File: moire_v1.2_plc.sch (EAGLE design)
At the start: 137 parts, among them IC1 TLC59281DBQ, IC11 LM4040B25, IC2 ROF-78E3.3-0.5SMD, IC3 4051PW, IC4 LM324PW, IC7 LD2981ABU33, IC9 LM324PW, J1 PJ301_THONKICONN6, J10 PJ301_THONKICONN6, J11 PJ301_THONKICONN6, J12 PJ301_THONKICONN6, J2 PJ301_THONKICONN6, J3 PJ301_THONKICONN6, J4 PJ301_THONKICONN6, J5 PJ301_THONKICONN6, J6 PJ301_THONKICONN6, J7 PJ301_THONKICONN6, J8 PJ301_THONKICONN6, J9 PJ301_THONKICONN6, Q2 8MHz, Q5 MMBT3904, Q6 MMBT3904, Q7 MMBT3904, U1 STM32F303K8T6, U2 MCP6004_SMD, U4 TL074_SMD

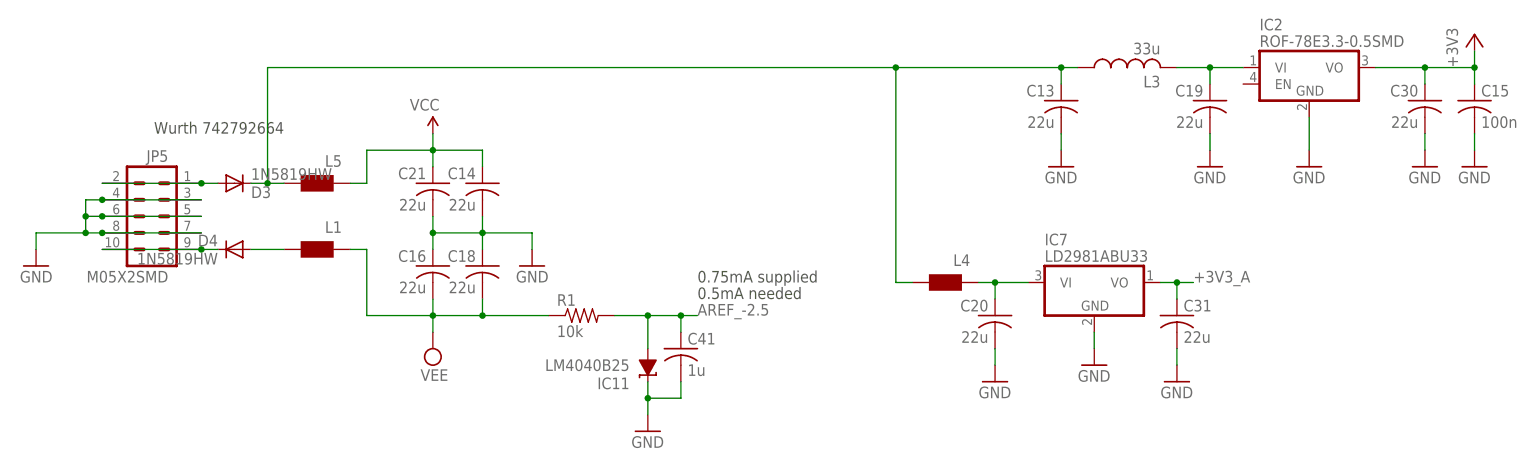
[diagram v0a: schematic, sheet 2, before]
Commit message: update brd
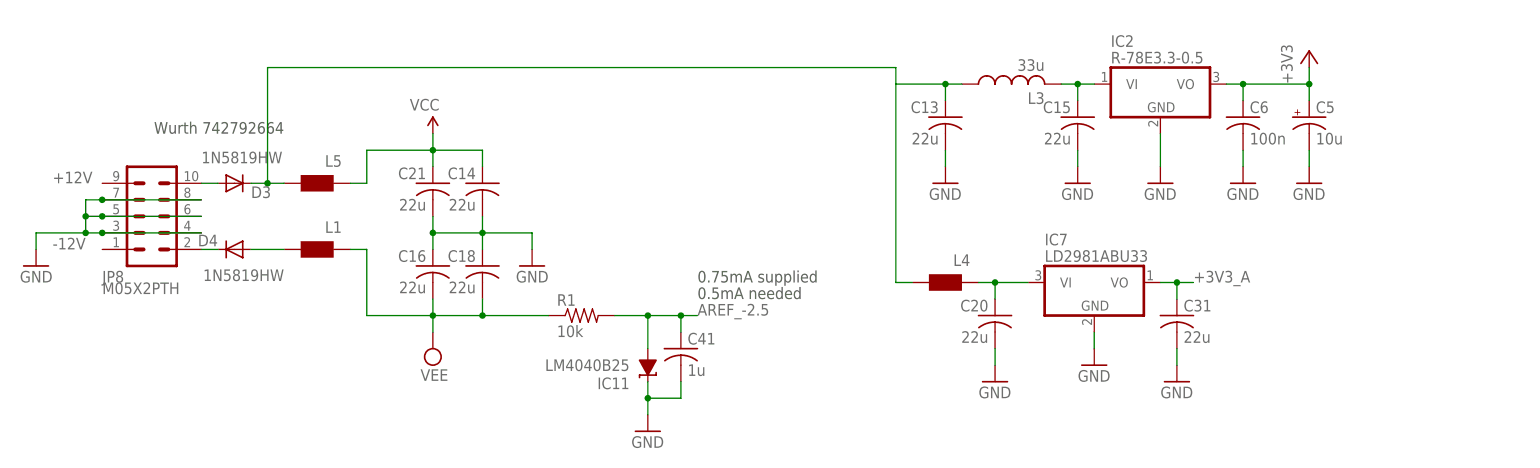
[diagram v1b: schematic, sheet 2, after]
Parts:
- removed C19, C30: 22u, rcl:C-USC1206
- removed IC4: LM324PW, og-linear:TL074PW
- removed JP5: M05X2SMD, og-header:M05X2SMD
- added C5: 10u, rcl:CPOL-USA
- added C6: 100n, rcl:C-USC0402
- added JP8: M05X2PTH, og-header:M05X2PTH
- C15: value 100n -> 22u; device rcl:C-USC0402 -> rcl:C-USC1206
- IC2: value ROF-78E3.3-0.5SMD -> R-78E3.3-0.5; device og-vreg:ROF-78EXX-0.55SMD -> og-vreg:WE173950378
- POT_A, POT_B, POT_C: device og-pots:POT_USVERTICAL_PS -> og-pots:POT_USVERTICAL
- R1, R10, R12, R13, R14, R16, R17, R20, R26, R28, R29, R4, R5, R51, R52, R53, R6, R66, R67, R68, R69, R70, R71, R8, R9: device rcl:R-US_R0402 -> rcl:R-US_R0603
- U$1: value ISL21010 -> VREF 1.5V
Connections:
- removed net N$18: D3.A, JP5.1, JP5.2
- removed net N$96: D4.C, JP5.10, JP5.9
- removed net N$99: C19.1, IC2.VI, L3.2
- new net +12V: D3.A, JP8.10, JP8.9
- new net -12V: D4.C, JP8.1, JP8.2
- new net N$66: C15.1, IC2.VI, L3.2
- new net N$67: C13.1, L3.1
- net +3V3: now also C5.+, C6.1; no longer C15.1, C30.1
- net GND: now also C5.-, C6.2, IC9P.V-, JP8.3, JP8.4, JP8.5, JP8.6, JP8.7, JP8.8; no longer C19.2, C30.2, IC4P.V-, JP5.3, JP5.4, JP5.5, JP5.6, JP5.7, JP5.8
- net N$4: no longer C13.1, L3.1
- net VCC: now also IC9P.V+; no longer IC4P.V+
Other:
- moved on the sheet: C13, C15, L3
